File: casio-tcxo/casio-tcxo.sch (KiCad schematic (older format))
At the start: 4 parts, among them U1 CASIO_ASIC, U2 SiT1552

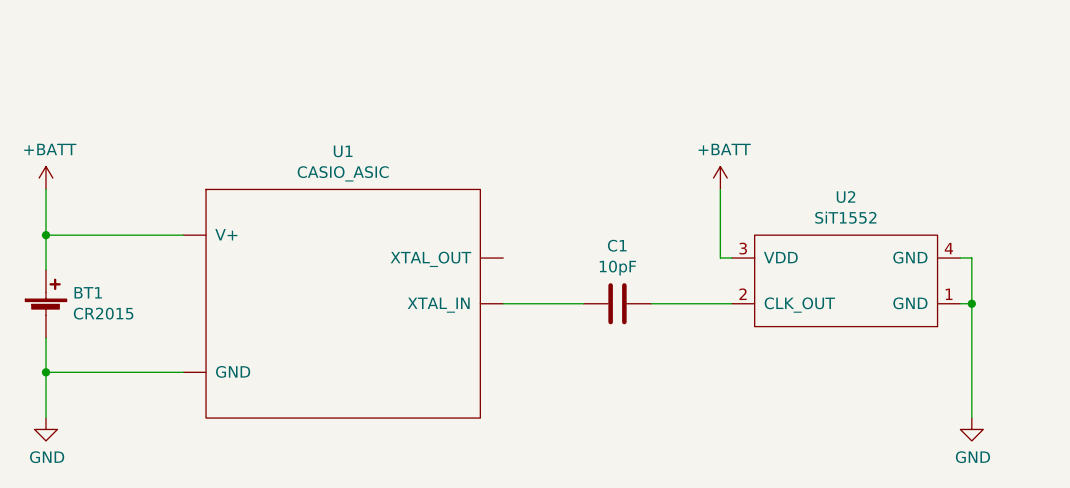
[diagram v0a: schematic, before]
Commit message: updated casio-tcxo
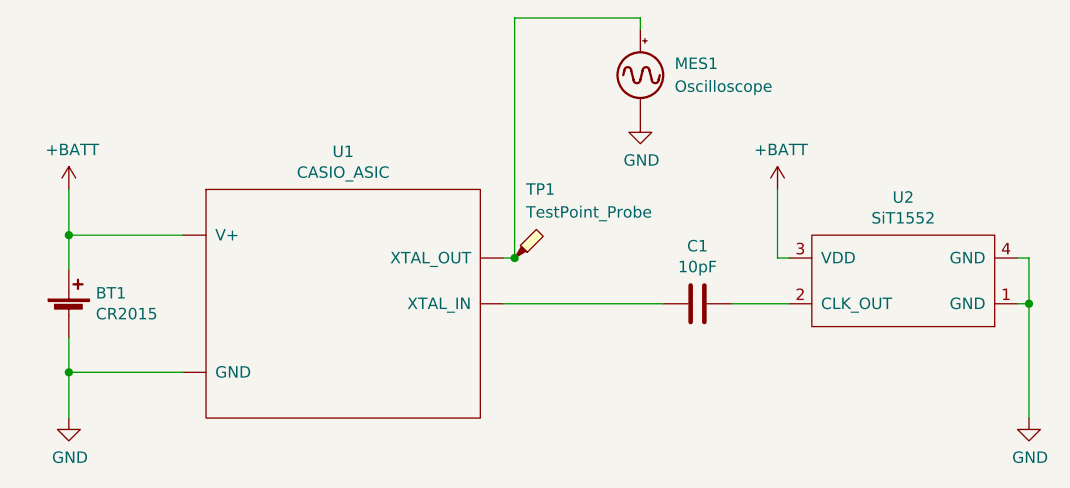
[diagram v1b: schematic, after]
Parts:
- added MES1: Oscilloscope, symbol Device:Oscilloscope
- added TP1: TestPoint_Probe, symbol Connector:TestPoint_Probe
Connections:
- net GND: now also MES1.1 (-)
- new net: MES1.2 (+), TP1.1, U1.~ (XTAL_OUT)
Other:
- moved on the sheet: BT1, C1, U2
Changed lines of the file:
@@
 L Device:C C1
 U 1 1 5E818B15
-P 4800 2600
-F 0 "C1" V 5052 2600 50  0000 C CNN
-F 1 "10pF" V 4961 2600 50  0000 C CNN
-F 2 "" H 4838 2450 50  0001 C CNN
-F 3 "~" H 4800 2600 50  0001 C CNN
-	1    4800 2600
+P 5150 2600
+F 0 "C1" V 5402 2600 50  0000 C CNN
+F 1 "10pF" V 5311 2600 50  0000 C CNN
+F 2 "" H 5188 2450 50  0001 C CNN
+F 3 "~" H 5150 2600 50  0001 C CNN
+	1    5150 2600
 	0    -1   -1   0
 $EndComp
@@
 L Device:Battery_Cell BT1
 U 1 1 5E81A6FF
-P 2300 2650
-F 0 "BT1" H 2418 2746 50  0000 L CNN
-F 1 "CR2015" H 2418 2655 50  0000 L CNN
-F 2 "" V 2300 2710 50  0001 C CNN
-F 3 "~" V 2300 2710 50  0001 C CNN
-	1    2300 2650
+P 2400 2650
+F 0 "BT1" H 2518 2746 50  0000 L CNN
+F 1 "CR2015" H 2518 2655 50  0000 L CNN
+F 2 "" V 2400 2710 50  0001 C CNN
+F 3 "~" V 2400 2710 50  0001 C CNN
+	1    2400 2650
 	1    0    0    -1
 $EndComp
@@
 L power:+BATT #PWR01
 U 1 1 5E81CD05
-P 2300 2100
-F 0 "#PWR01" H 2300 1950 50  0001 C CNN
-F 1 "+BATT" H 2315 2273 50  0000 C CNN
-F 2 "" H 2300 2100 50  0001 C CNN
-F 3 "" H 2300 2100 50  0001 C CNN
-	1    2300 2100
+P 2400 2100
+F 0 "#PWR01" H 2400 1950 50  0001 C CNN
+F 1 "+BATT" H 2415 2273 50  0000 C CNN
+F 2 "" H 2400 2100 50  0001 C CNN
+F 3 "" H 2400 2100 50  0001 C CNN
+	1    2400 2100
 	1    0    0    -1
 $EndComp
@@
 L power:+BATT #PWR04
 U 1 1 5E81DB05
-P 5250 2100
-F 0 "#PWR04" H 5250 1950 50  0001 C CNN
-F 1 "+BATT" H 5265 2273 50  0000 C CNN
-F 2 "" H 5250 2100 50  0001 C CNN
-F 3 "" H 5250 2100 50  0001 C CNN
-	1    5250 2100
+P 5500 2100
+F 0 "#PWR04" H 5500 1950 50  0001 C CNN
+F 1 "+BATT" H 5515 2273 50  0000 C CNN
+F 2 "" H 5500 2100 50  0001 C CNN
+F 3 "" H 5500 2100 50  0001 C CNN
+	1    5500 2100
 	1    0    0    -1
 $EndComp
@@
 L power:GND #PWR02
 U 1 1 5E821DD8
-P 2300 3100
-F 0 "#PWR02" H 2300 2850 50  0001 C CNN
-F 1 "GND" H 2305 2927 50  0000 C CNN
-F 2 "" H 2300 3100 50  0001 C CNN
-F 3 "" H 2300 3100 50  0001 C CNN
-	1    2300 3100
+P 2400 3100
+F 0 "#PWR02" H 2400 2850 50  0001 C CNN
+F 1 "GND" H 2405 2927 50  0000 C CNN
+F 2 "" H 2400 3100 50  0001 C CNN
+F 3 "" H 2400 3100 50  0001 C CNN
+	1    2400 3100
 	1    0    0    -1
 $EndComp
 Wire Wire Line
-	2300 3100 2300 2900
+	2400 3100 2400 2900
 Wire Wire Line
-	2300 2100 2300 2300
+	2400 2100 2400 2300
 Wire Wire Line
-	2900 2300 2300 2300
-Connection ~ 2300 2300
+	2900 2300 2400 2300
+Connection ~ 2400 2300
 Wire Wire Line
-	2300 2300 2300 2450
+	2400 2300 2400 2450
 Wire Wire Line
-	2900 2900 2300 2900
-Connection ~ 2300 2900
+	2900 2900 2400 2900
+Connection ~ 2400 2900
 Wire Wire Line
-	2300 2900 2300 2750
+	2400 2900 2400 2750
 Wire Wire Line
-	4300 2600 4650 2600
+	4300 2600 5000 2600
 Wire Wire Line
-	4950 2600 5300 2600
+	5300 2600 5550 2600
 $Comp
 L power:GND #PWR05
 U 1 1 5E82BADB
-P 6350 3100
-F 0 "#PWR05" H 6350 2850 50  0001 C CNN
-F 1 "GND" H 6355 2927 50  0000 C CNN
-F 2 "" H 6350 3100 50  0001 C CNN
-F 3 "" H 6350 3100 50  0001 C CNN
-	1    6350 3100
+P 6600 3100
+F 0 "#PWR05" H 6600 2850 50  0001 C CNN
+F 1 "GND" H 6605 2927 50  0000 C CNN
+F 2 "" H 6600 3100 50  0001 C CNN
+F 3 "" H 6600 3100 50  0001 C CNN
+	1    6600 3100
 	1    0    0    -1
 $EndComp
@@
 L microfarad-de:SiT1552 U2
 U 1 1 5E8380E8
-P 5800 2500
-F 0 "U2" H 5800 2135 50  0000 C CNN
-F 1 "SiT1552" H 5800 2226 50  0000 C CNN
-F 2 "" H 5800 2500 50  0001 C CNN
-F 3 "" H 5800 2500 50  0001 C CNN
-	1    5800 2500
+P 6050 2500
+F 0 "U2" H 6050 2135 50  0000 C CNN
+F 1 "SiT1552" H 6050 2226 50  0000 C CNN
+F 2 "" H 6050 2500 50  0001 C CNN
+F 3 "" H 6050 2500 50  0001 C CNN
+	1    6050 2500
 	-1   0    0    1
 $EndComp
 Wire Wire Line
-	6350 3100 6350 2600
+	6600 3100 6600 2600
 Wire Wire Line
-	6350 2400 6300 2400
+	6600 2400 6550 2400
 Wire Wire Line
-	6300 2600 6350 2600
-Connection ~ 6350 2600
+	6550 2600 6600 2600
+Connection ~ 6600 2600
 Wire Wire Line
-	6350 2600 6350 2400
+	6600 2600 6600 2400
 Wire Wire Line
-	5250 2100 5250 2400
+	5500 2100 5500 2400
 Wire Wire Line
-	5250 2400 5300 2400
+	5500 2400 5550 2400
+$Comp
+L Device:Oscilloscope MES1
+U 1 1 5E83ABF3
+P 4900 1600
+F 0 "MES1" H 5050 1650 50  0000 L CNN
+F 1 "Oscilloscope" H 5050 1550 50  0000 L CNN
+F 2 "" V 4900 1700 50  0001 C CNN
+F 3 "~" V 4900 1700 50  0001 C CNN
+	1    4900 1600
+	1    0    0    -1
+$EndComp
+$Comp
+L power:GND #PWR03
+U 1 1 5E8543D1
+P 4900 1800
+F 0 "#PWR03" H 4900 1550 50  0001 C CNN
+F 1 "GND" H 4905 1627 50  0000 C CNN
+F 2 "" H 4900 1800 50  0001 C CNN
+F 3 "" H 4900 1800 50  0001 C CNN
+	1    4900 1800
+	1    0    0    -1
+$EndComp
+$Comp
+L Connector:TestPoint_Probe TP1
+U 1 1 5E85A702
+P 4350 2400
+F 0 "TP1" H 4400 2700 50  0000 L CNN
+F 1 "TestPoint_Probe" H 4400 2600 50  0000 L CNN
+F 2 "" H 4550 2400 50  0001 C CNN
+F 3 "~" H 4550 2400 50  0001 C CNN
+	1    4350 2400
+	1    0    0    -1
+$EndComp
+Wire Wire Line
+	4300 2400 4350 2400
+Wire Wire Line
+	4350 2400 4350 1350
+Wire Wire Line
+	4350 1350 4900 1350
+Wire Wire Line
+	4900 1350 4900 1400
+Connection ~ 4350 2400
 $EndSCHEMATC
